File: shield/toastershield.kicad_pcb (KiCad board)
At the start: 2 copper layers, 68.6 x 53.3 mm, 33 parts, among them J1 Power, J2 Digital/PWM, J3 Analog, J4 Digital/PWM, SW1 SW_SPDT, SW2 SW_SPDT, SW3 SW_SPDT, SW4 SW_SPDT, U2 NE555P, U3 74HC14

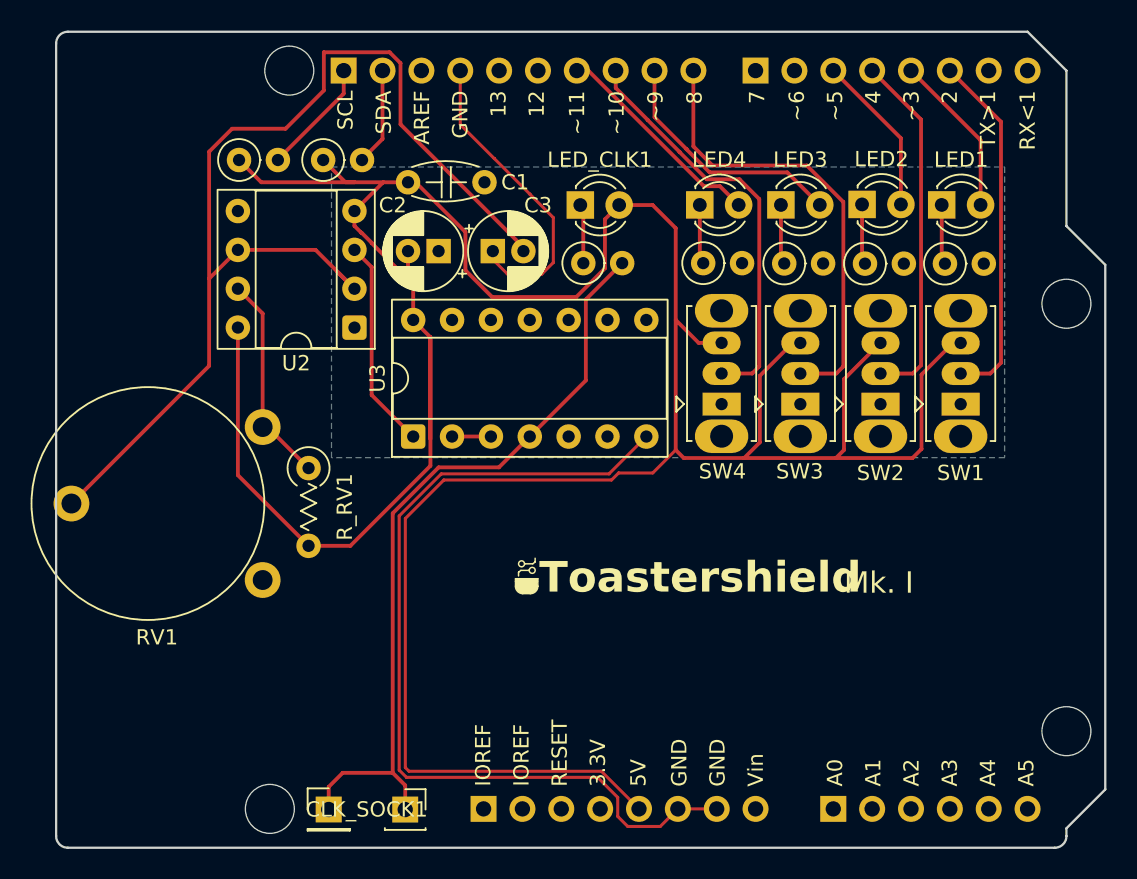
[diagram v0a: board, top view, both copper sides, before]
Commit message: feat: fix text and pins
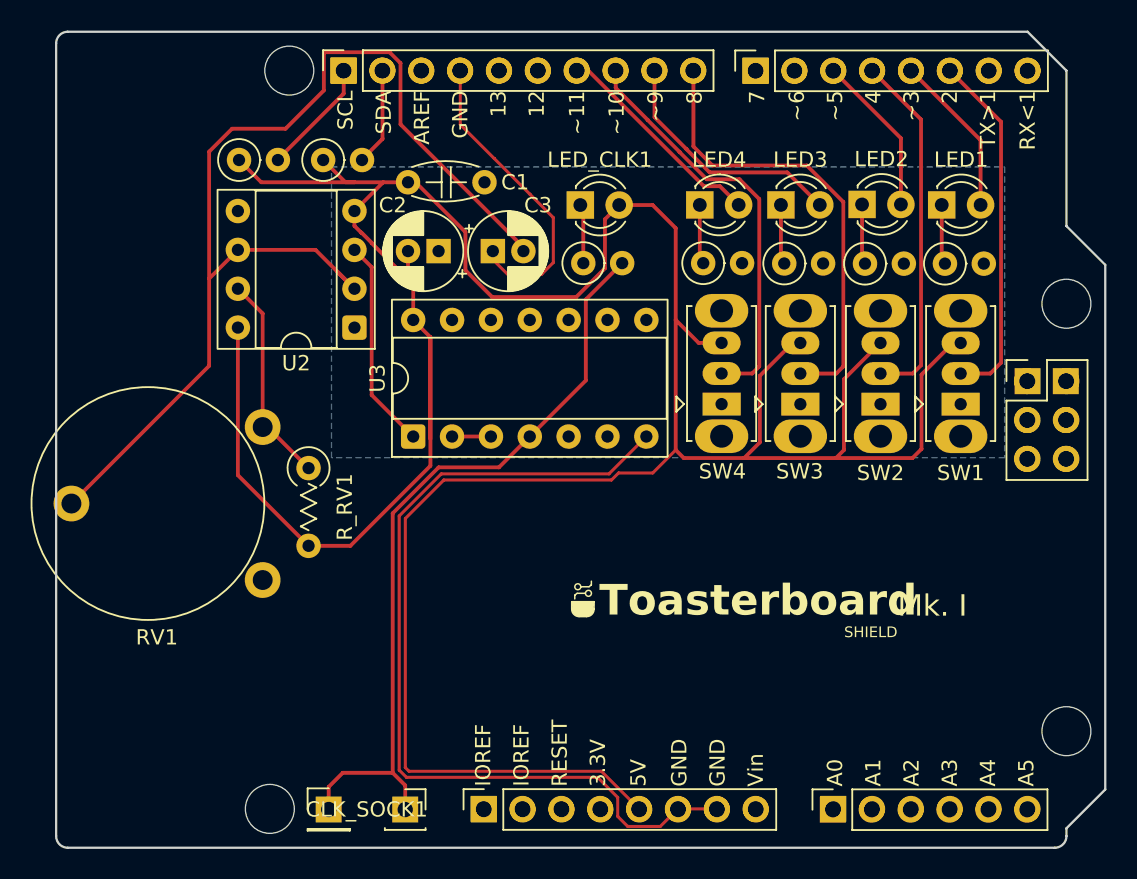
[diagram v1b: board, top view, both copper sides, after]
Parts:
- added J5: PinHeader_2x03_P2.54mm_Vertical, Connector_PinHeader_2.54mm:PinHeader_2x03_P2.54mm_Vertical, B.Cu at (166.0, 69.5)
- added JB1: PinSocket_1x08_P2.54mm_Vertical, Connector_PinSocket_2.54mm:PinSocket_1x08_P2.54mm_Vertical, F.Cu at (128.0, 97.5)
- added JB2: PinSocket_1x10_P2.54mm_Vertical, Connector_PinSocket_2.54mm:PinSocket_1x10_P2.54mm_Vertical, F.Cu at (118.8, 49.2)
- added JB3: PinSocket_1x06_P2.54mm_Vertical, Connector_PinSocket_2.54mm:PinSocket_1x06_P2.54mm_Vertical, F.Cu at (150.8, 97.5)
- added JB4: PinSocket_1x08_P2.54mm_Vertical, Connector_PinSocket_2.54mm:PinSocket_1x08_P2.54mm_Vertical, F.Cu at (145.7, 49.2)
- added JB5: PinHeader_2x03_P2.54mm_Vertical, Connector_PinHeader_2.54mm:PinHeader_2x03_P2.54mm_Vertical, F.Cu at (163.5, 69.5)
- J1, J4: footprint Connector_PinSocket_2.54mm:PinSocket_1x08_P2.54mm_Vertical -> Connector_PinHeader_2.54mm:PinHeader_1x08_P2.54mm_Vertical
- J2: footprint Connector_PinSocket_2.54mm:PinSocket_1x10_P2.54mm_Vertical -> Connector_PinHeader_2.54mm:PinHeader_1x10_P2.54mm_Vertical
- J3: footprint Connector_PinSocket_2.54mm:PinSocket_1x06_P2.54mm_Vertical -> Connector_PinHeader_2.54mm:PinHeader_1x06_P2.54mm_Vertical
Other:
- board text added: "SHIELD"
- board text added: "Toasterboard"
- board text removed: "Toastershield"
